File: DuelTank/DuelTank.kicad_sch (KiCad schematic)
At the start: 70 parts, among them J1 AudioJack, J2 Speaker, J3 1053131105, J4 Pot, J5 1053131105, J6 GND, J7 DACOUT, SW1 Shield, SW2 Fire, SW3 Left, SW4 Right, U2 LP-MSPM0G3507, U3 MCP34119P, U4 HiLetGo_ST7735R, U5 ULN2003B, U6 TSOP31438

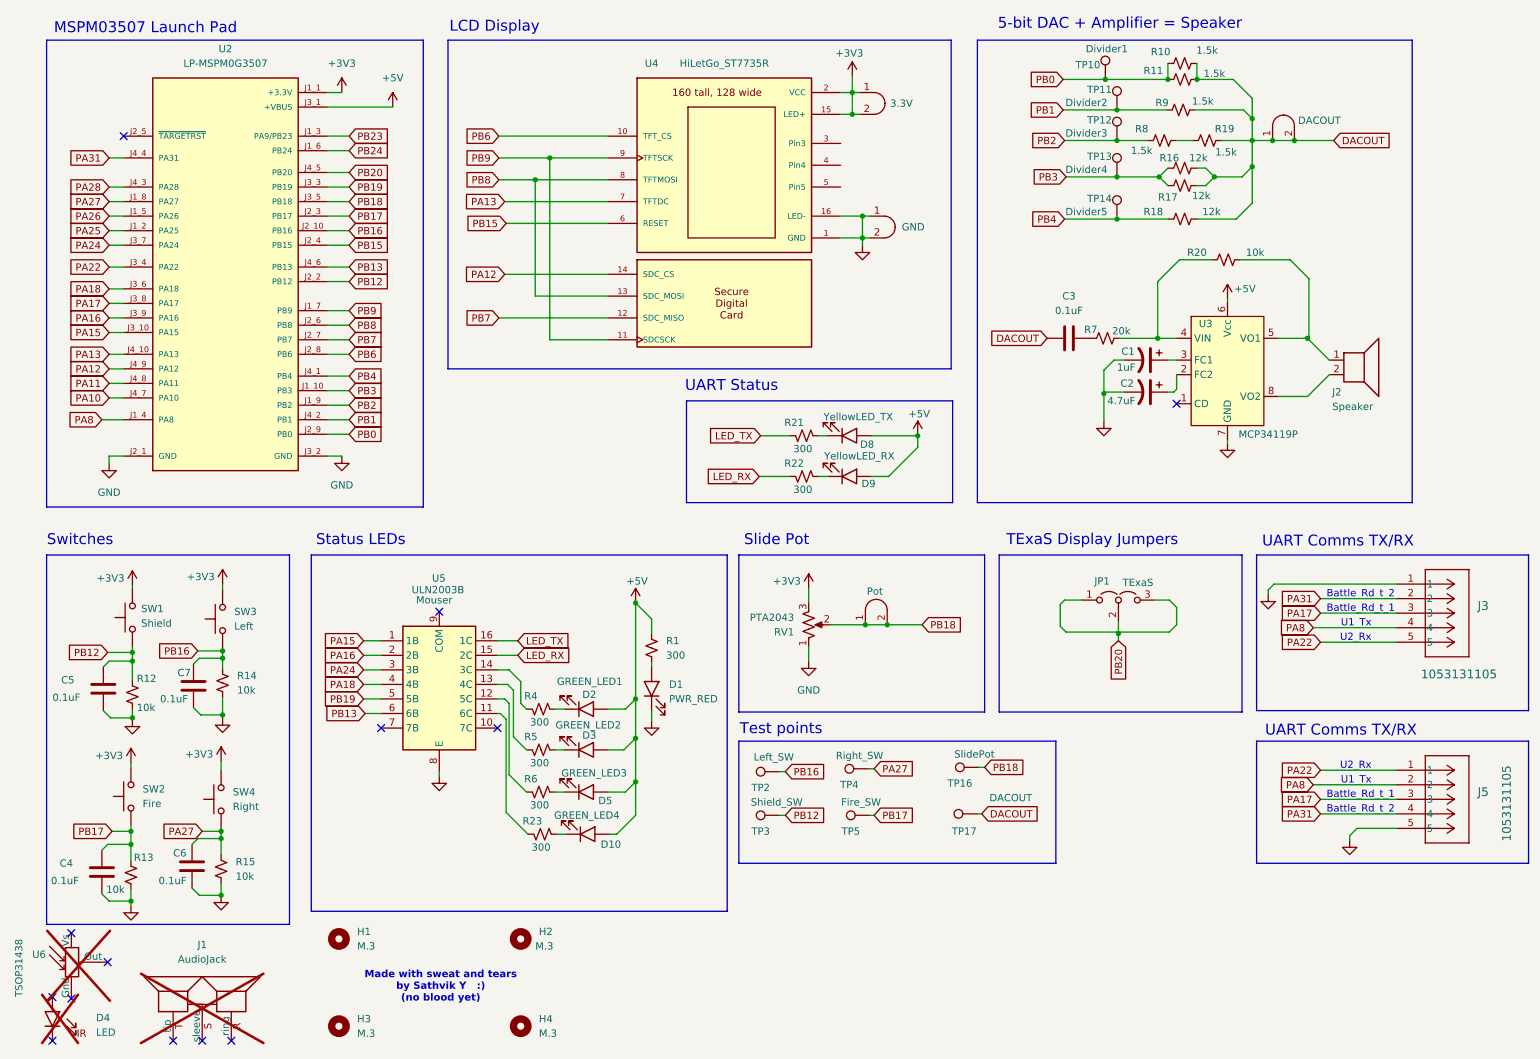
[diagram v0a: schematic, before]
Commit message: board ordered!
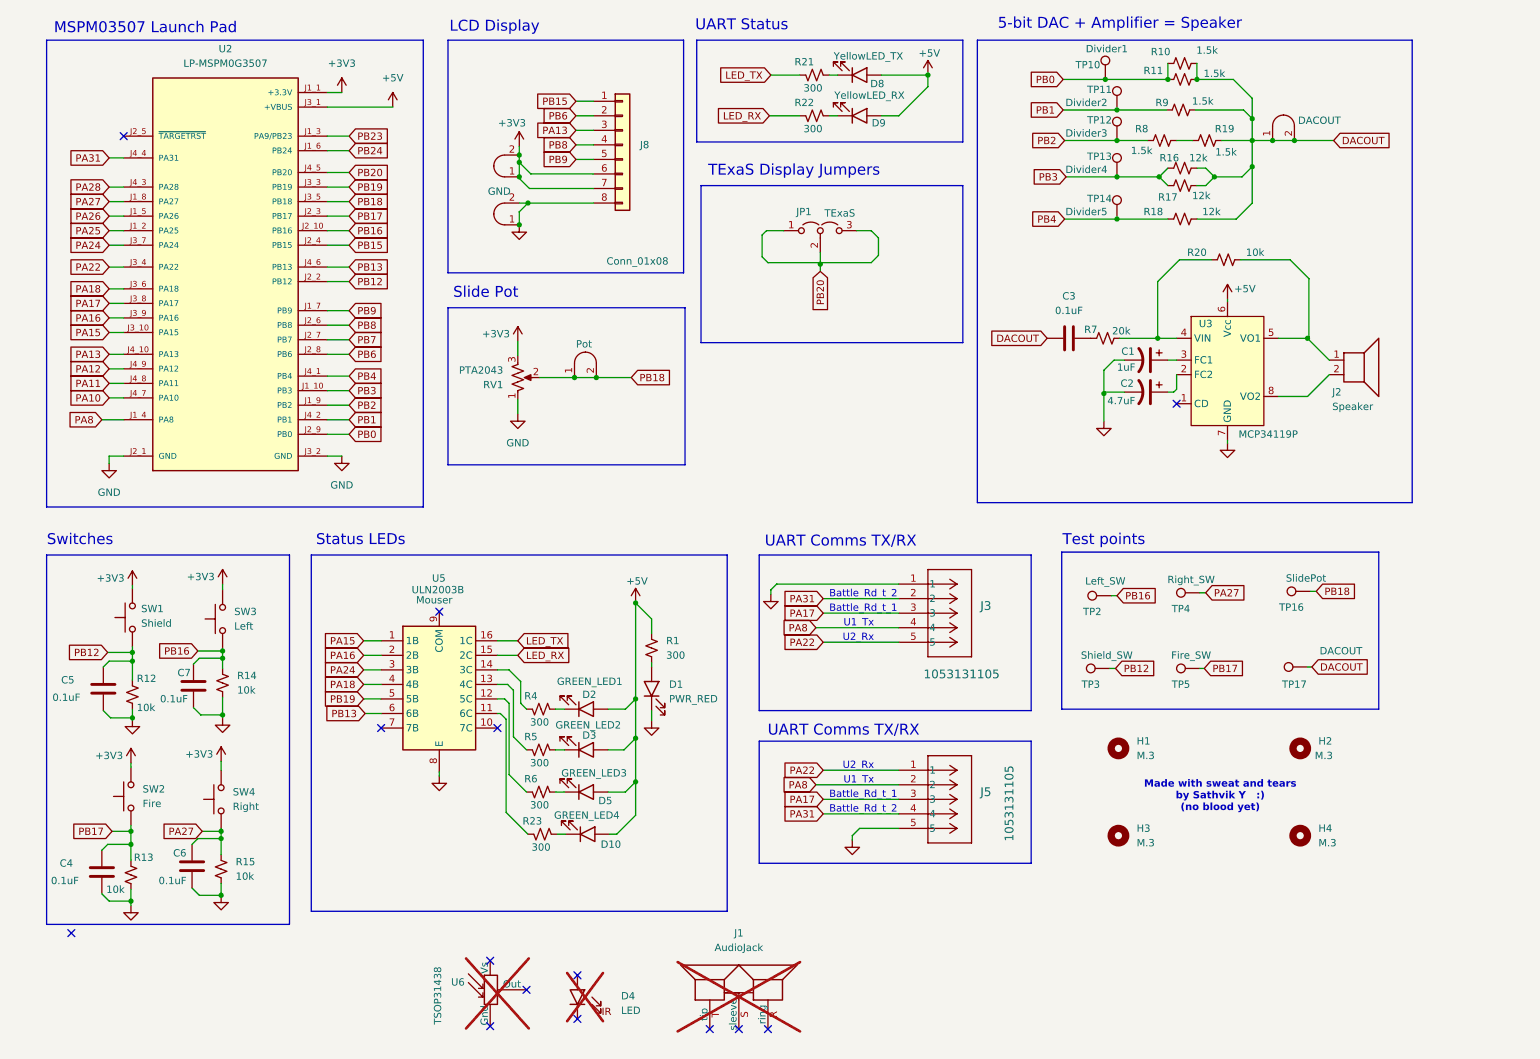
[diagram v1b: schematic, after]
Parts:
- removed U4: HiLetGo_ST7735R, ECE319K:hiletgo_st7735r, symbol ECE319K:HiLetGo_ST7735R
- added J8: Conn_01x08, Connector_PinHeader_2.54mm:PinHeader_1x08_P2.54mm_Vertical, symbol Connector_Generic:Conn_01x08
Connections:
- net +3V3: now also J8.6 (Pin_6), J8.7 (Pin_7)
- net GND: now also J8.8 (Pin_8)
- net PA13: now also J8.3 (Pin_3)
- net PB15: now also J8.1 (Pin_1)
- net PB6: now also J8.2 (Pin_2)
- net PB8: now also J8.4 (Pin_4)
- net PB9: now also J8.5 (Pin_5)
- no-connect marks 13 -> 14
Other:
- moved on the sheet: D4, D8, D9, H1, H2, H3, H4, J1, J3, J5, JP1, R21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
